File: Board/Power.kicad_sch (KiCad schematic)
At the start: 90 parts, among them J15 2171800001

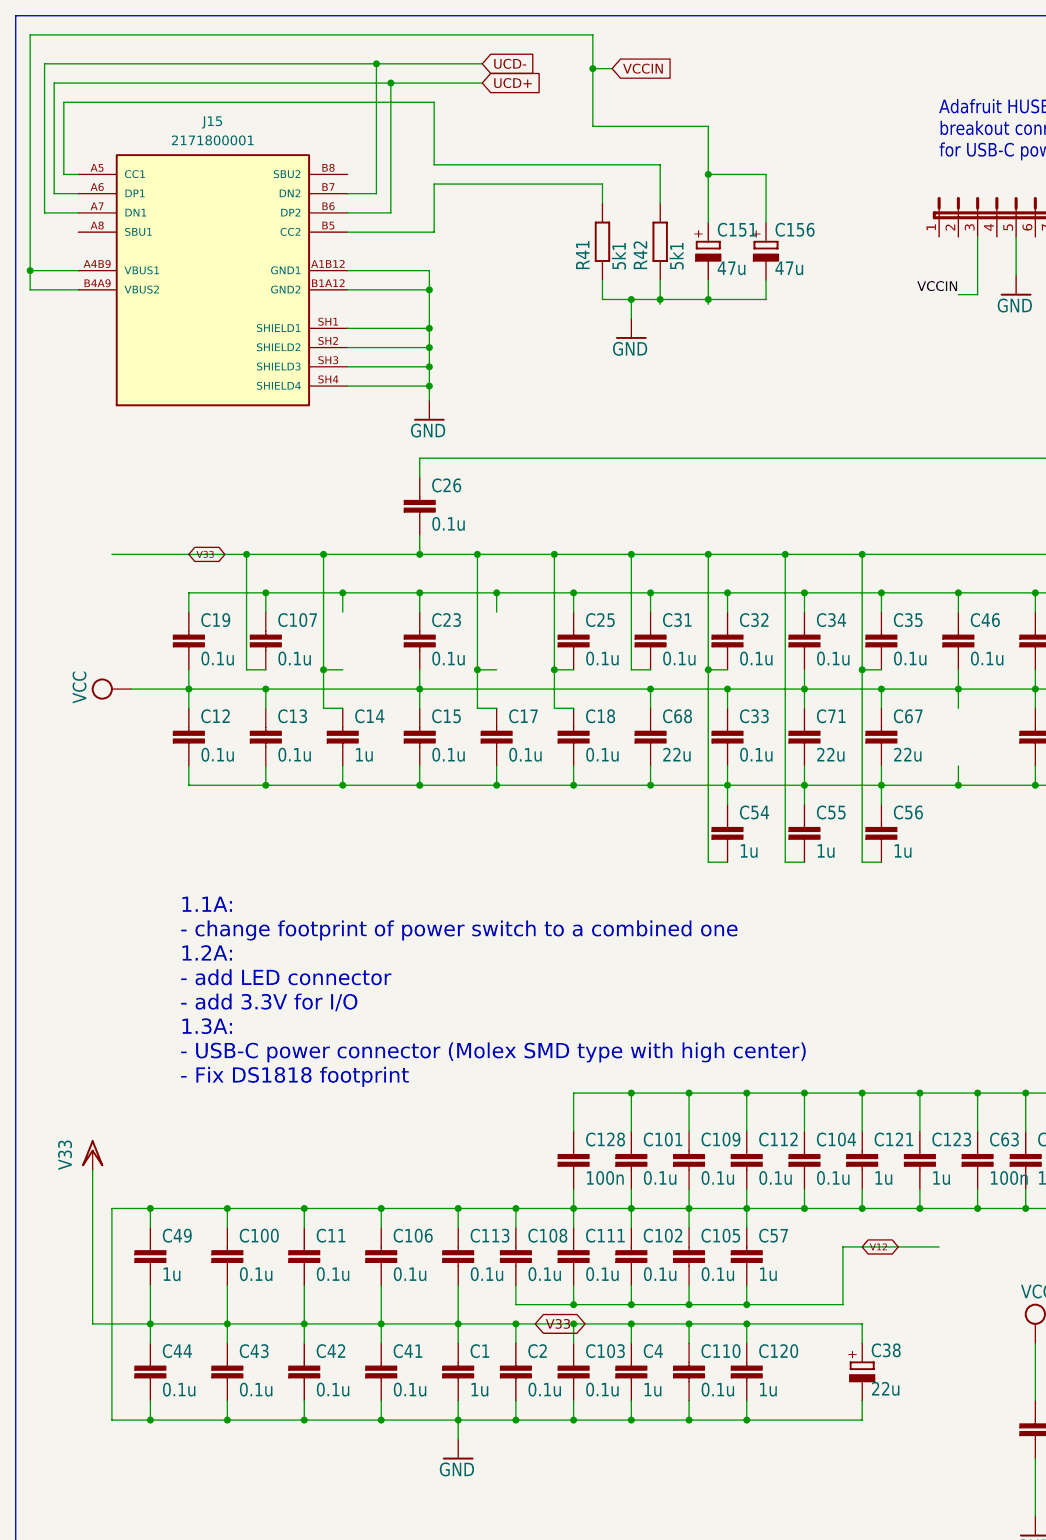
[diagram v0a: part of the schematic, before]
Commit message: some layout fixes, more parts
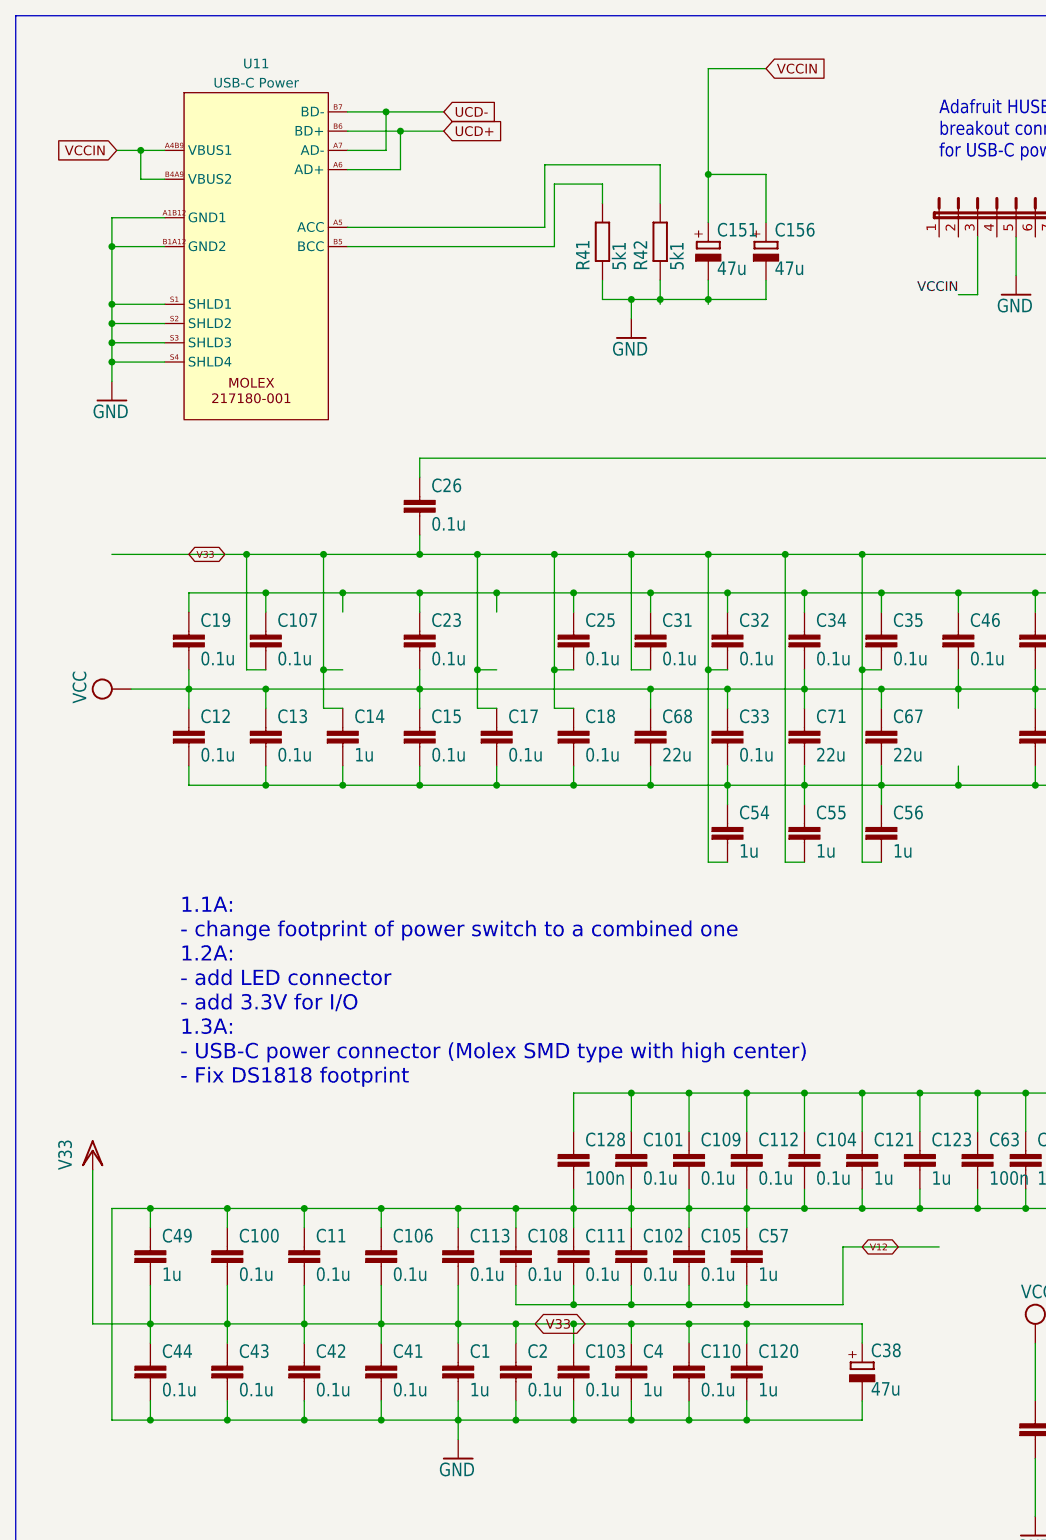
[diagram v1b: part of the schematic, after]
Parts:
- removed J15: 2171800001, cbm_ultipet_v1:MOLEX_2171800001, symbol Symbols:2171800001
- added U11: USB-C Power, cbm_ultipet_v1:USB-C-217180, symbol Symbols:USB-C-217180
- C38: value 22u -> 47u
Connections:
- net GND: now also U11.A1B12 (GND1), U11.B1A12 (GND2), U11.S1 (SHLD1), U11.S2 (SHLD2), U11.S3 (SHLD3), U11.S4 (SHLD4)
- net UCD+: now also U11.A6 (AD+), U11.B6 (BD+)
- net UCD-: now also U11.A7 (AD-), U11.B7 (BD-)
- net VCCIN: now also U11.A4B9 (VBUS1), U11.B4A9 (VBUS2)
- net at R42.2: now also U11.A5 (ACC)
- net at R41.2: now also U11.B5 (BCC)
